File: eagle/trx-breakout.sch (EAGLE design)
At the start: 9 parts, among them J1 DF12NB(3.0)-10DX-0.5VHRS_DF12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, Q1 BSS84, Q2 BSS84, Q3 BSS123, Q4 BSS123

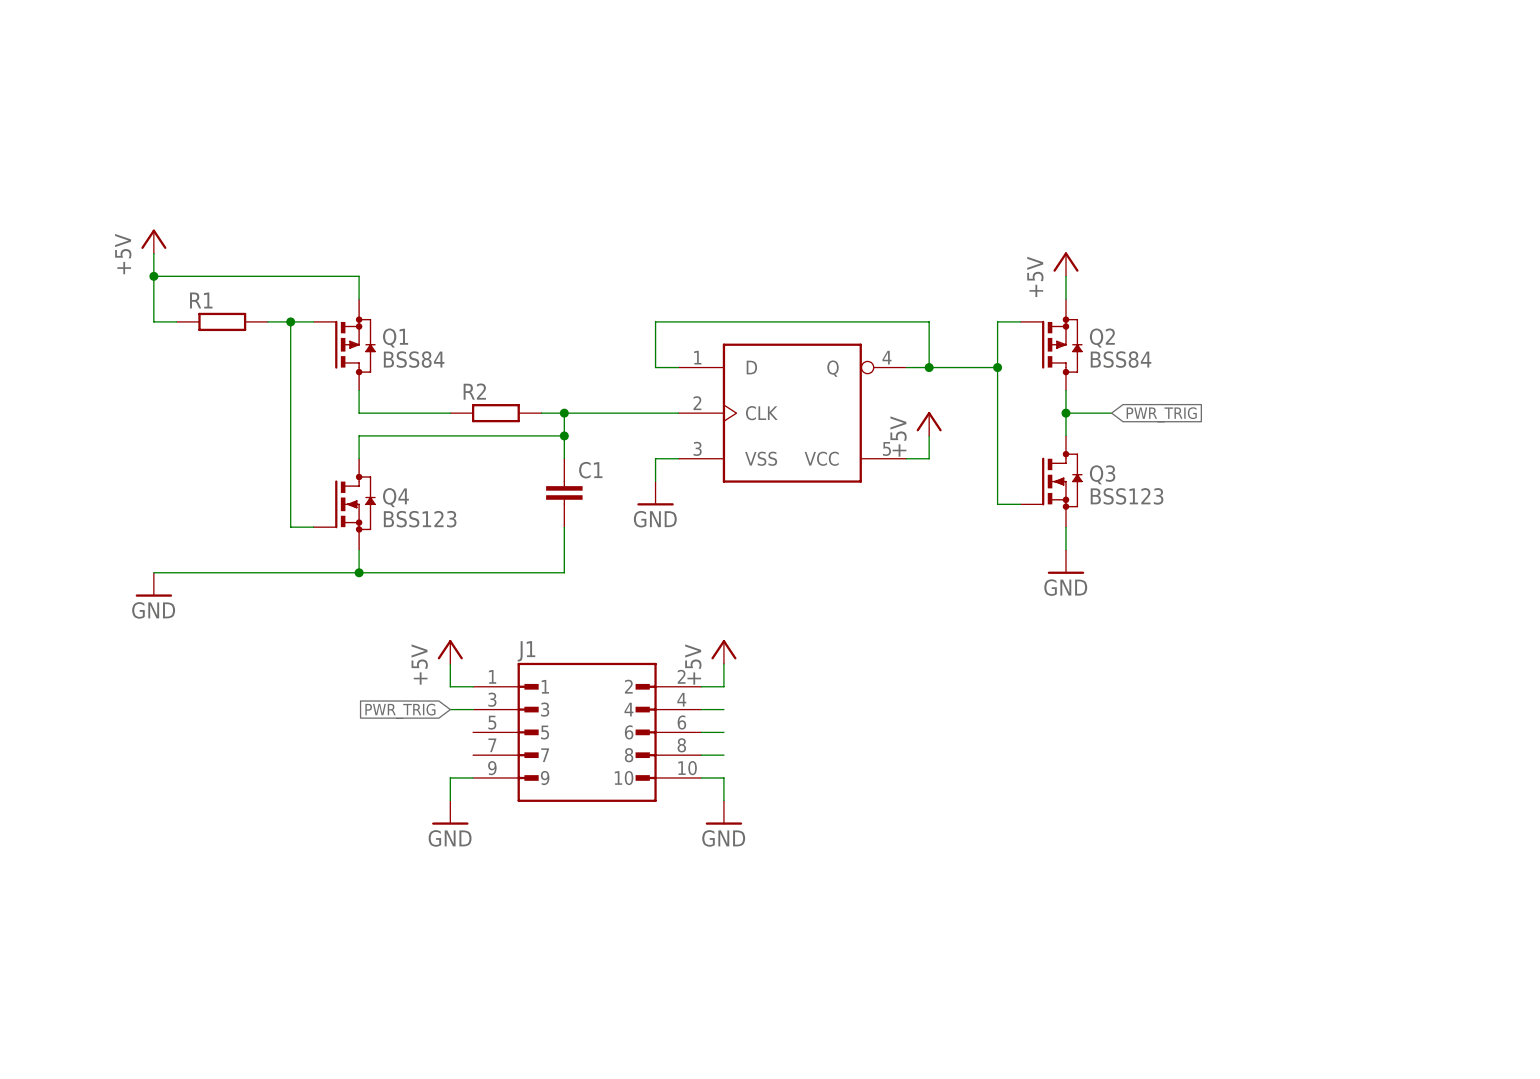
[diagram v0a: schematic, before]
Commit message: Finalized alpha design
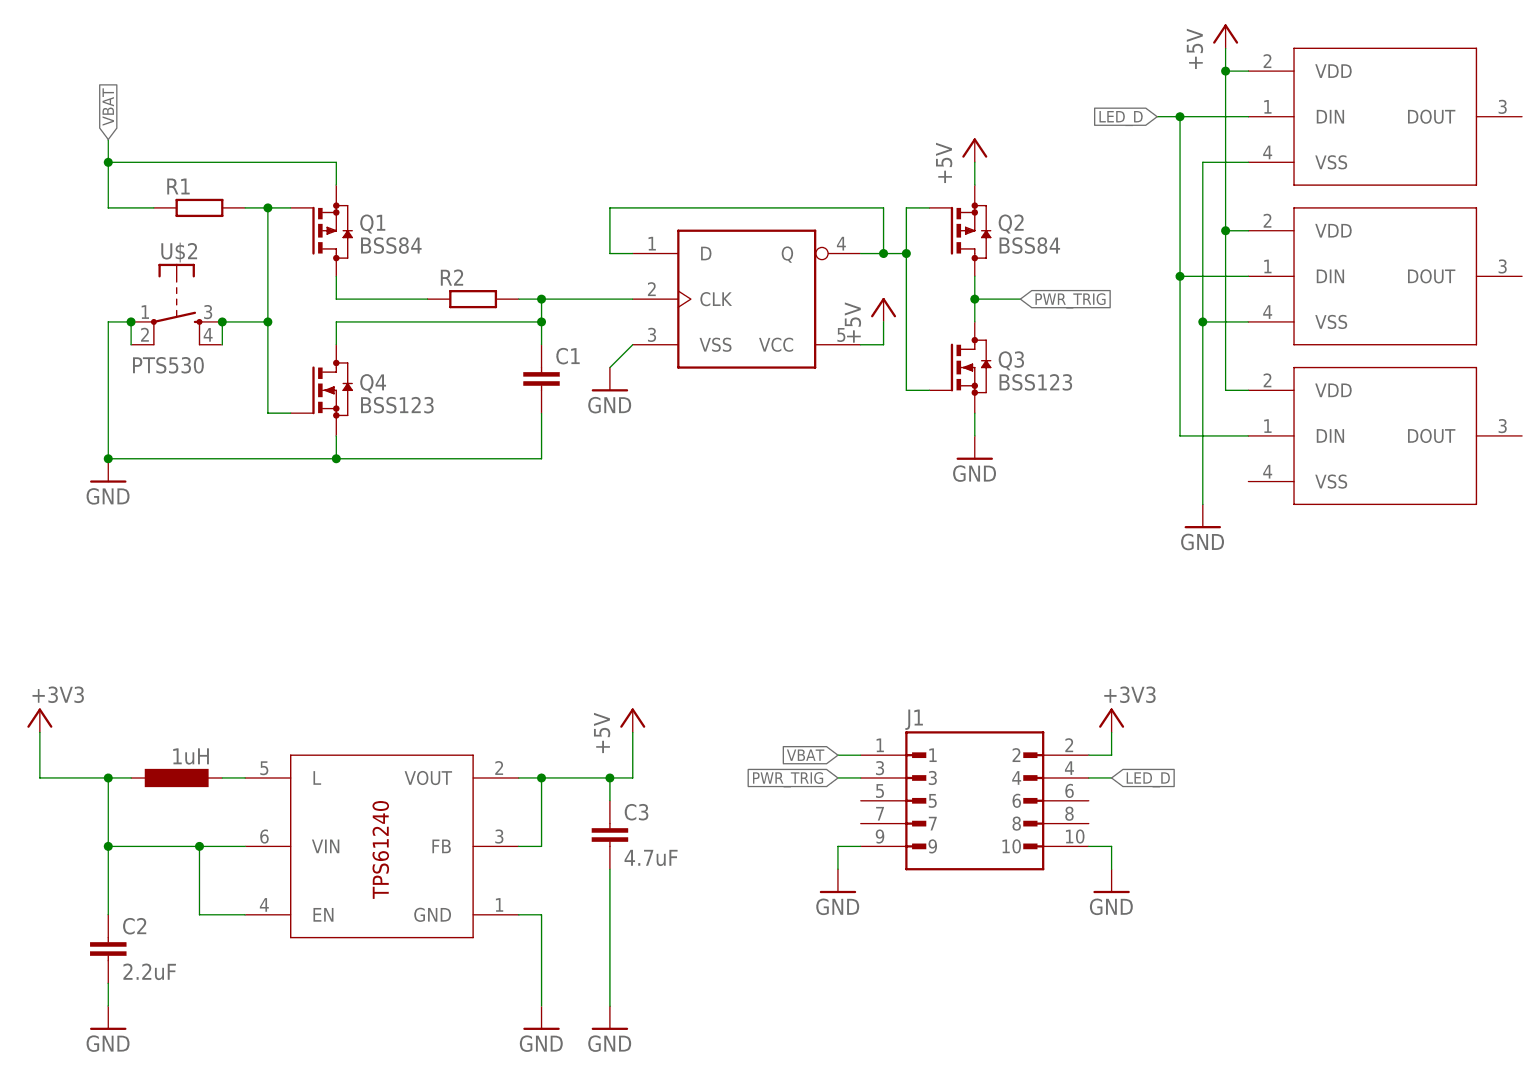
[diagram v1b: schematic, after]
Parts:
- added C2: 2.2uF, rcl:C-EUC0805
- added C3: 4.7uF, rcl:C-EUC0805
- added U$2: PTS530, switches-ck:PTS530
- added U$3: TPS61240, texas-instruments:TPS61240
- added U$4: 1uH, inductor-vishay:IHLP-1212
- added U$5, U$6, U$7: ARGB_LED, led:ARGB_LED
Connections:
- removed net N$10: J1.8
- removed net N$8: J1.4
- removed net N$9: J1.6
- new net +3V3: C2.1, J1.2, U$3.EN, U$3.VIN, U$4.1
- new net LED_D: J1.4, U$5.DIN, U$6.DIN, U$7.DIN
- new net N$6: Q1.G, Q4.G, R1.2, U$2.S, U$2.S@1
- new net VBAT: J1.1, Q1.S, R1.1
- net +5V: now also C3.1, U$3.FB, U$3.VOUT, U$5.VDD, U$6.VDD, U$7.VDD; no longer J1.1, J1.2, Q1.S, R1.1
- net GND: now also C2.2, C3.2, U$2.P, U$2.P@1, U$3.GND, U$5.VSS, U$6.VSS
- net N$1: now also U$3.L, U$4.2; no longer Q1.G, Q4.G, R1.2
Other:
- moved on the sheet: C1, J1, Q1, Q2, Q3, Q4, R1, R2
